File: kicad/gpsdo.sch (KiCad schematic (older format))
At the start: 54 parts, among them J1 Conn_Coaxial, J2 Conn_01x04_Male, J3 Conn_01x04_Male, J4 Conn_01x04_Male, J5 Conn_01x04_Male, J6 Conn_01x04_Male, U1 MSP430F5171IDA, U10 74AUC1G79, U11 47L64, U12 47L64, U2 MAX-8Q, U3 549CAAC000111BBG, U4 Si7051-A20, U5 LTC4317, U6 74LVC1G08, U7 74LVC1G08, U8 74AUC1G79, U9 74LVC1G86

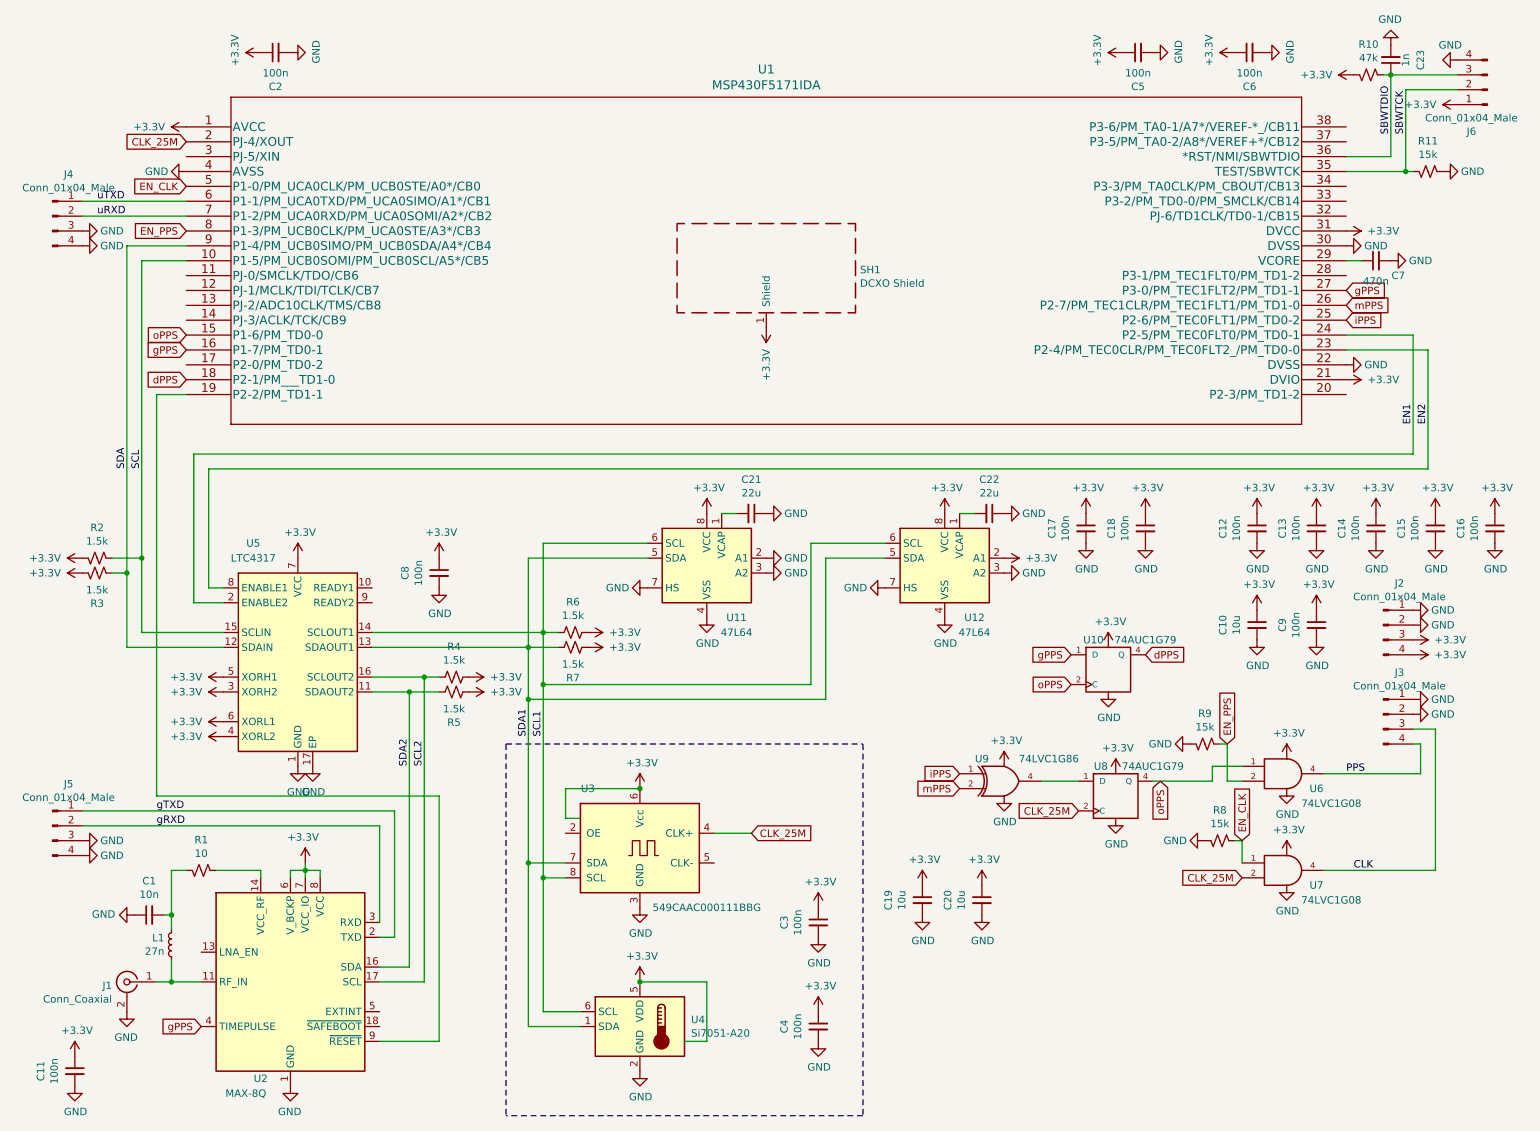
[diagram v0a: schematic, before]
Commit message: update pcb layout
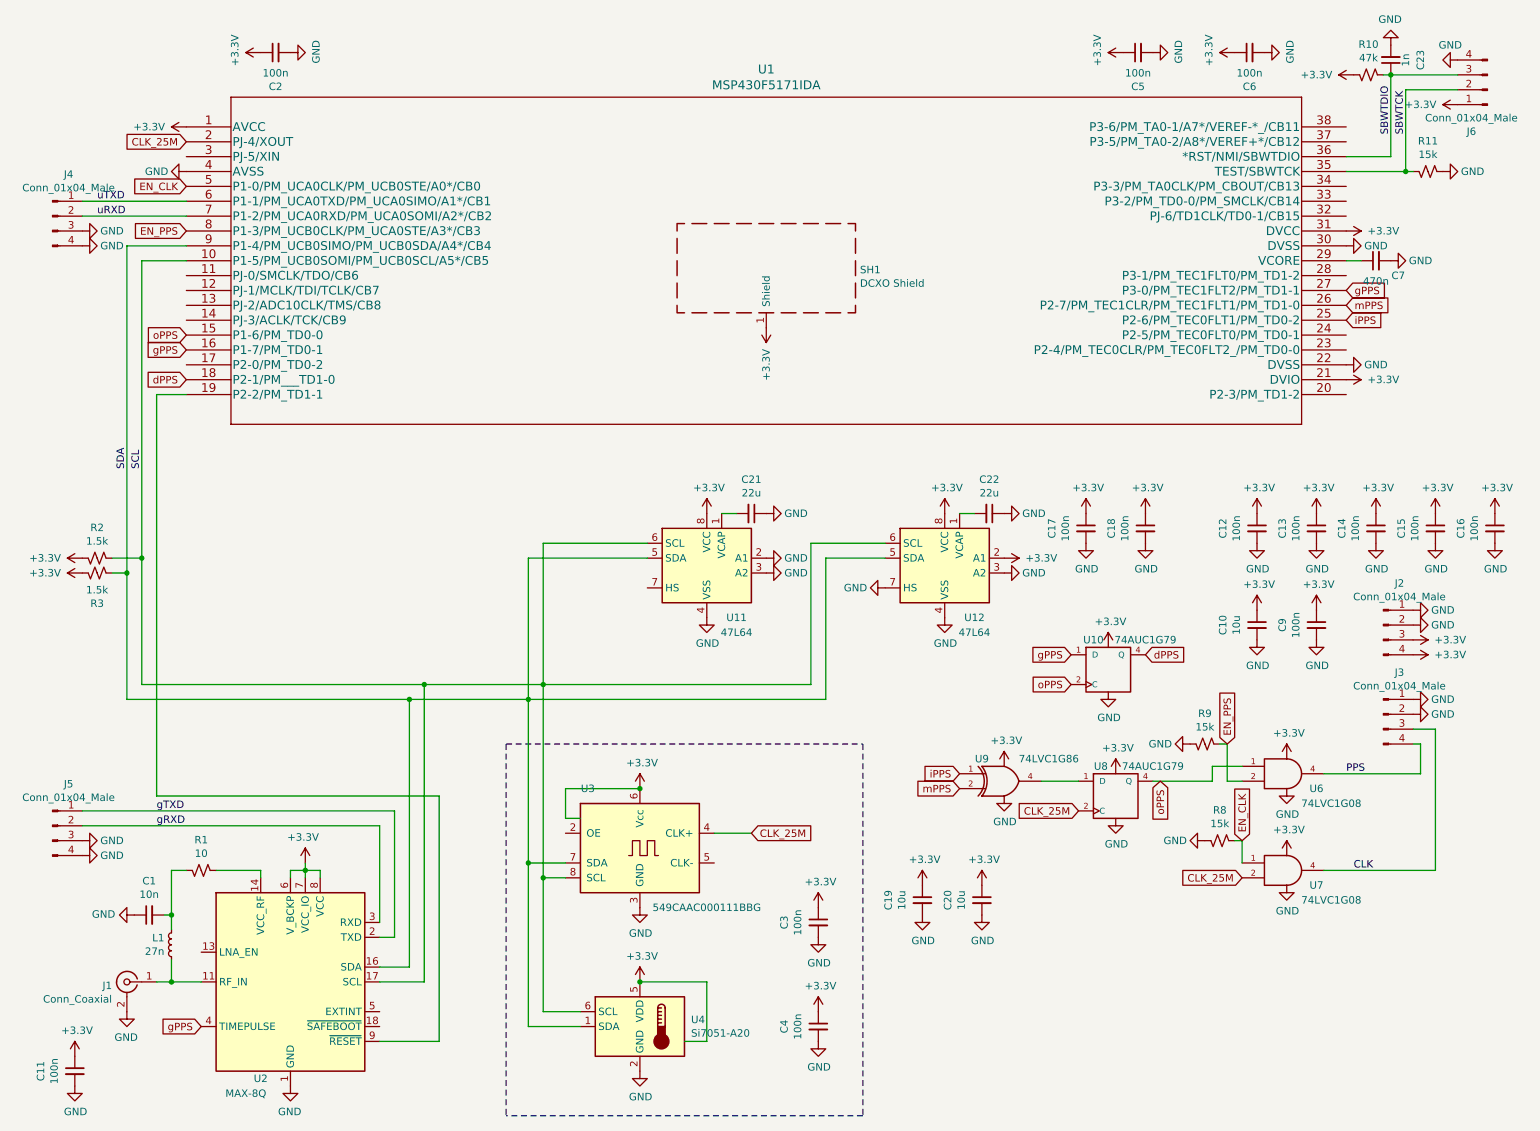
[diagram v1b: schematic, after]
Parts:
- removed C8: 100n, Resistor_SMD:R_0603_1608Metric, symbol Device:C_Small
- removed R4, R5, R6, R7: 1.5k, Resistor_SMD:R_0603_1608Metric, symbol Device:R_Small_US
- removed U5: LTC4317, Package_DFN_QFN:DFN-16-1EP_3x5mm_P0.5mm_EP1.66x4.4mm, symbol Interface:LTC4317
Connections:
- net SCL1 is gone; now on net SCL: U11.6 (SCL), U12.6 (SCL), U3.8 (SCL), U4.6 (SCL)
- net SCL2 is gone; now on net SCL: U2.17 (SCL)
- net SDA1 is gone; now on net SDA: U11.5 (SDA), U12.5 (SDA), U3.7 (SDA), U4.1 (SDA)
- net SDA2 is gone; now on net SDA: U2.16 (SDA)
- net GND: no longer U11.7 (HS)
- net EN1: no longer names the net of U1.24 (P2-5/PM_TEC0FLT0/PM_TD0-1)
- net EN2: no longer names the net of U1.23 (P2-4/PM_TEC0CLR/PM_TEC0FLT2_/PM_TD0-0)
